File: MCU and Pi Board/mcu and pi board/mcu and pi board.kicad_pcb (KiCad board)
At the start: 4 copper layers, 141.1 x 213.2 mm, 100 parts, among them IC3 CSD17578Q3A, IC4 CSD17578Q3A, J1 PJ-002A, J10 ET60T-D04-0-00-D04-X-R1-S, J11 Conn_02x13_Odd_Even, J12 430450428, J13 IPBT-105-H1-T-D-GP, J14 IPBT-105-H1-T-D-GP, J15 Conn_01x28_Socket, J16 Conn_01x28_Socket, J17 DebugnBoot, J18 UART-PINS, J2 ET60S-D04-3-08-D04-X-R1-S, J22 Conn_01x03_Pin, J23 TB006-508-03BE, J24 TB006-508-03BE, J25 TB006-508-03BE, J3 BM04B-GHS-TBT, J4 PJ-002A, J5 Conn_02x20_Odd_Even, J6 Conn_01x04_Socket, J7 Conn_01x04_Pin, J8 PWM Connector, J9 ESC ADAPTER - BACKPLANE, Q1 BSC010N04LS6ATMA1, Q2 BSC010N04LS6ATMA1, U1 STM32F091CCT6, U2 LM3940IMPX-3.3/NOPB, U3 LTC4370CMS_PBF, U4 TPS40305DRCR, U5 RASPBERRY_PI_4B_4GB, U6 MC74HC157ADR2G, U7 MC74HC157ADR2G

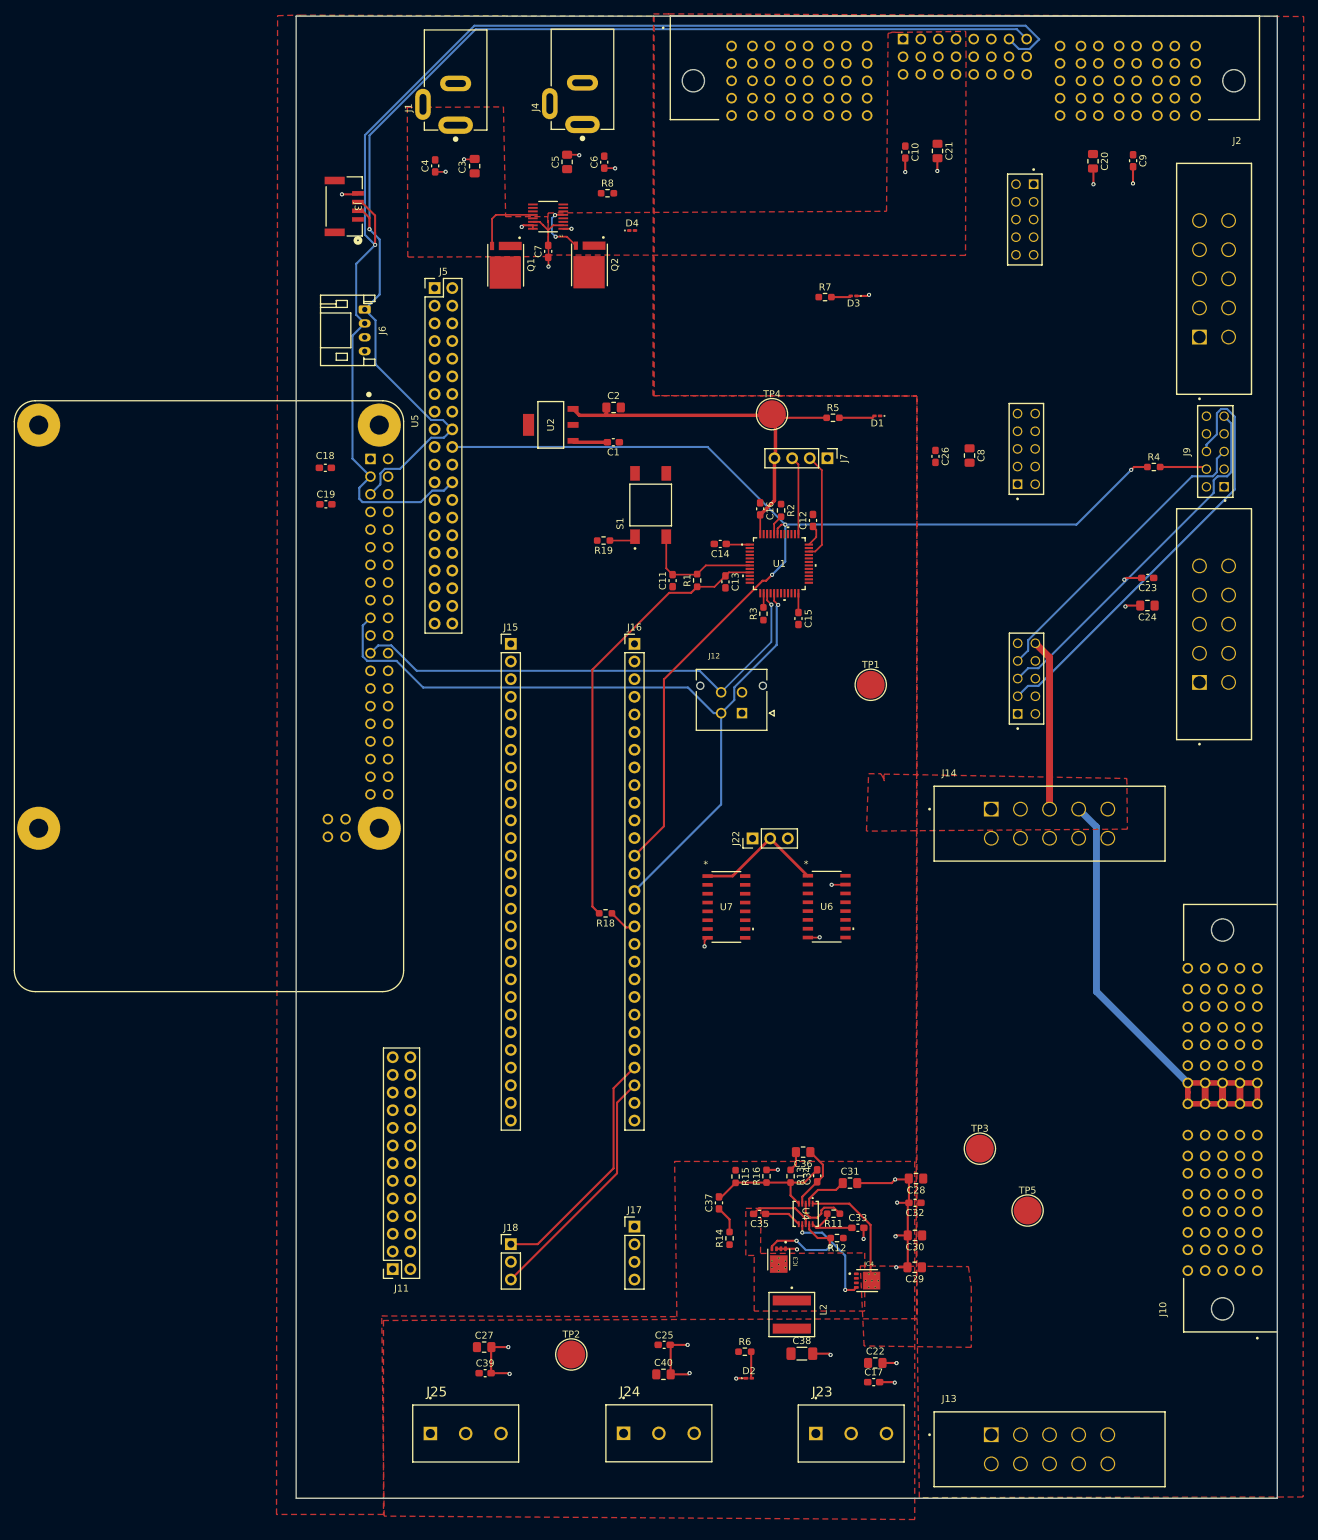
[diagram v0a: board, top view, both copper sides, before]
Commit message: yeet
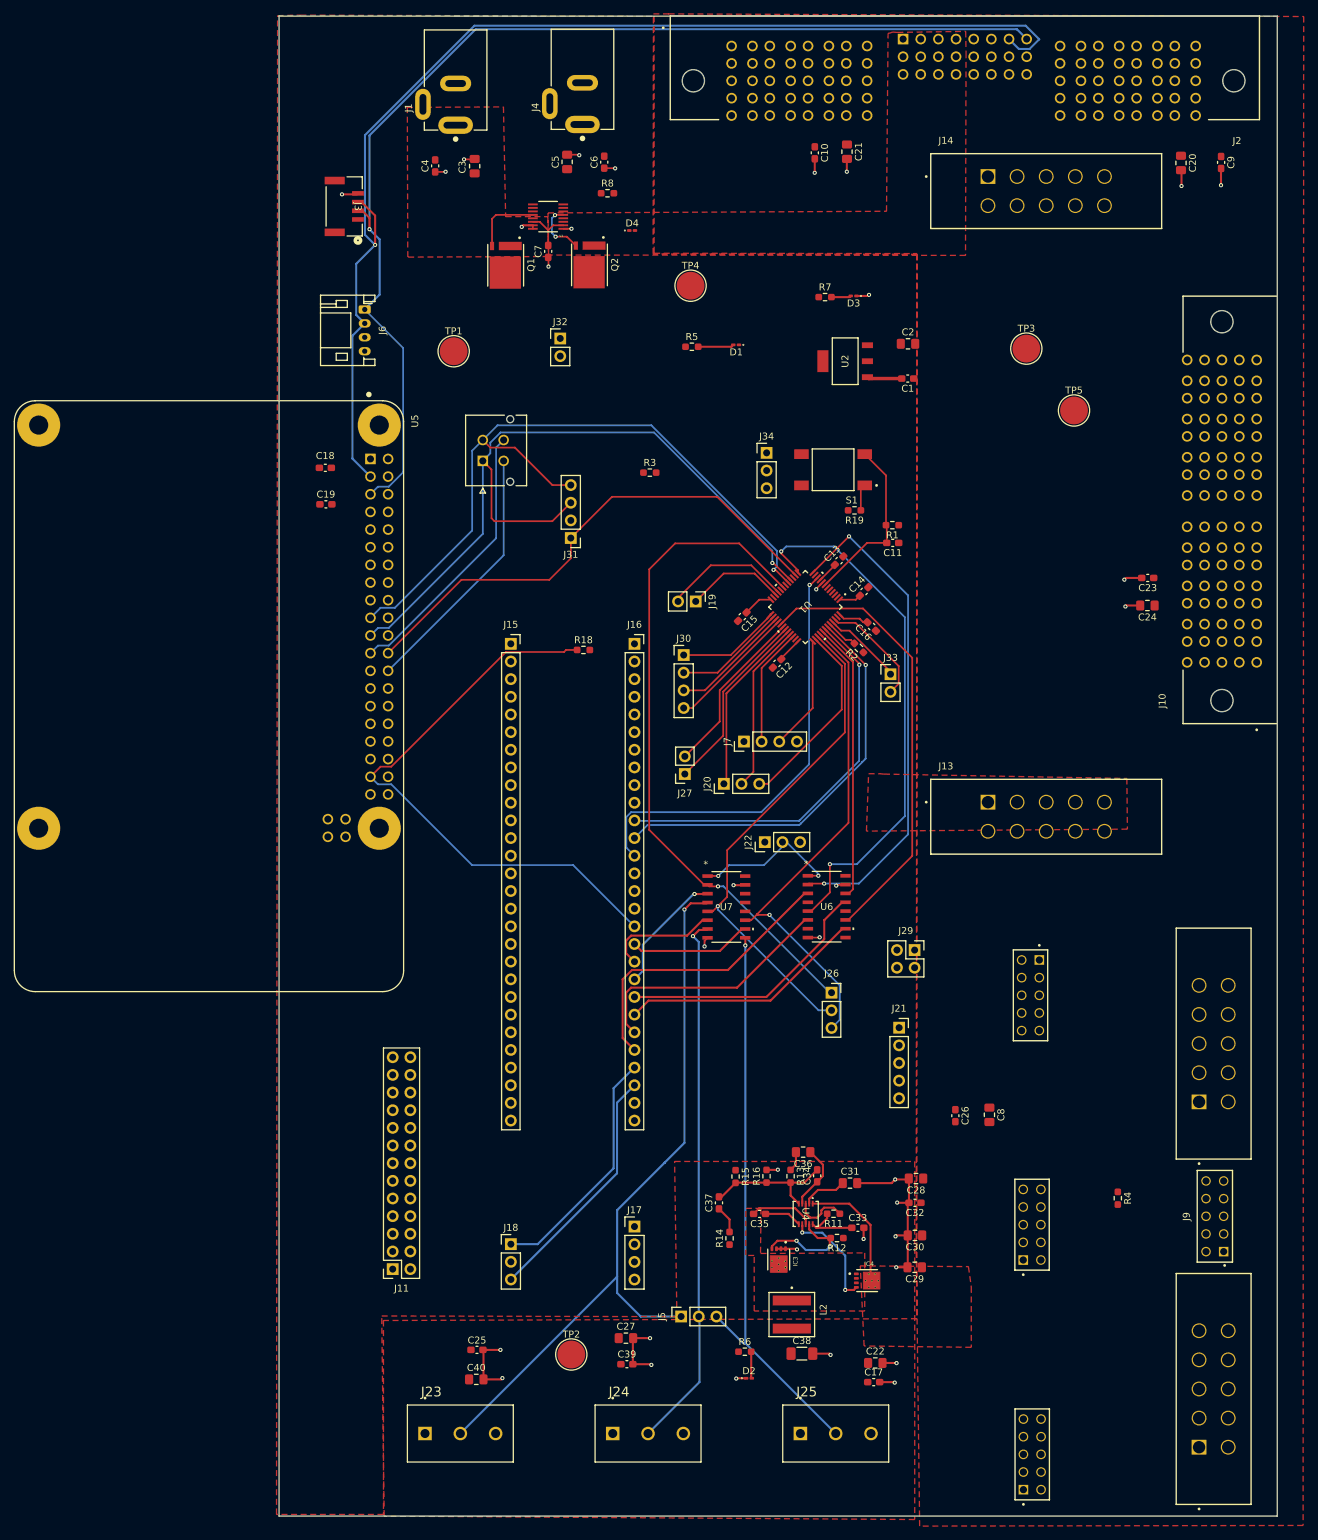
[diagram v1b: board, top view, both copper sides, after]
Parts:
- added J19: Conn_01x02_Pin, Connector_PinHeader_2.54mm:PinHeader_1x02_P2.54mm_Vertical, F.Cu at (218.9, 112.3)
- added J20: Conn_01x03_Pin, Connector_PinHeader_2.54mm:PinHeader_1x03_P2.54mm_Vertical, F.Cu at (223.0, 138.5)
- added J21: Conn_01x05, Connector_PinSocket_2.54mm:PinSocket_1x05_P2.54mm_Vertical, F.Cu at (248.2, 173.6)
- added J26: Conn_01x03_Pin, Connector_PinSocket_2.54mm:PinSocket_1x03_P2.54mm_Vertical, F.Cu at (238.5, 168.6)
- added J27: Conn_01x02_Pin, Connector_PinSocket_2.54mm:PinSocket_1x02_P2.54mm_Vertical, F.Cu at (217.4, 137.1)
- added J29: Conn_02x02_Pin, Connector_PinSocket_2.54mm:PinSocket_2x02_P2.54mm_Vertical, F.Cu at (250.4, 162.4)
- added J30: Conn_01x04_Pin, Connector_PinHeader_2.54mm:PinHeader_1x04_P2.54mm_Vertical, F.Cu at (217.2, 120.0)
- added J31: Conn_01x04_Pin, Connector_PinHeader_2.54mm:PinHeader_1x04_P2.54mm_Vertical, F.Cu at (201.0, 103.2)
- added J32: Conn_01x02_Pin, Connector_PinHeader_2.54mm:PinHeader_1x02_P2.54mm_Vertical, F.Cu at (199.4, 74.5)
- added J33: Conn_01x02_Pin, Connector_PinHeader_2.54mm:PinHeader_1x02_P2.54mm_Vertical, F.Cu at (247.0, 122.8)
- added J34: Conn_01x03_Pin, Connector_PinHeader_2.54mm:PinHeader_1x03_P2.54mm_Vertical, F.Cu at (229.1, 90.9)
- J15, J16: footprint Connector_PinHeader_2.54mm:PinHeader_1x28_P2.54mm_Vertical -> Connector_PinSocket_2.54mm:PinSocket_1x28_P2.54mm_Vertical
- J5: value Conn_02x20_Odd_Even -> Conn_01x03_Pin; footprint Connector_PinHeader_2.54mm:PinHeader_2x20_P2.54mm_Vertical -> Connector_PinSocket_2.54mm:PinSocket_1x03_P2.54mm_Vertical
- TP1, TP2: value 6V -> TestPoint
- TP4: value 3.3V -> TestPoint
- moved J5 152.1 mm to (216.8, 215.2), turned to 90 degrees
- moved TP3 115.3 mm to (266.5, 75.9)
- moved TP5 115.3 mm to (273.4, 84.8)
- moved J8 111.6 mm to (267.3, 202.0)
- moved J9 110.0 mm to (293.5, 200.8)
- moved R4 105.3 mm to (279.7, 198.2), turned to -90 degrees
- moved C26 94.9 mm to (256.3, 186.3)
- moved C8 94.9 mm to (261.2, 186.2)
- moved J13 91.0 mm to (269.4, 143.3)
- moved J14 91.0 mm to (269.4, 53.3)
- moved J10 87.5 mm to (294.6, 99.3)
- moved TP1 76.8 mm to (184.1, 76.3)
- moved J23 56.2 mm to (180.0, 232.0)
- moved J25 53.2 mm to (234.0, 232.0)
- moved J12 52.0 mm to (188.3, 92.1), turned to -90 degrees
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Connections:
- J10 pad P03_1: +12V -> GND
- J10 pad P03_10: +12V -> GND
- J10 pad P03_2: +12V -> GND
- J10 pad P03_3: +12V -> GND
- J10 pad P03_4: +12V -> GND
- J10 pad P03_5: +12V -> GND
- J10 pad P03_6: +12V -> GND
- J10 pad P03_7: +12V -> GND
- J10 pad P03_8: +12V -> GND
- J10 pad P03_9: +12V -> GND
- J10 pad P04_1: +12V -> GND
- J10 pad P04_10: +12V -> GND
- J10 pad P04_2: +12V -> GND
- J10 pad P04_3: +12V -> GND
- J10 pad P04_4: +12V -> GND
- J10 pad P04_5: +12V -> GND
- J10 pad P04_6: +12V -> GND
- J10 pad P04_7: +12V -> GND
- J10 pad P04_8: +12V -> GND
- J10 pad P04_9: +12V -> GND
- J10 pad P07_1: GND -> +12V
- J10 pad P07_10: GND -> +12V
- J10 pad P07_2: GND -> +12V
- J10 pad P07_3: GND -> +12V
- J10 pad P07_4: GND -> +12V
- J10 pad P07_5: GND -> +12V
- J10 pad P07_6: GND -> +12V
- J10 pad P07_7: GND -> +12V
- J10 pad P07_8: GND -> +12V
- J10 pad P07_9: GND -> +12V
- J10 pad P08_1: GND -> +12V
- J10 pad P08_10: GND -> +12V
- J10 pad P08_2: GND -> +12V
- J10 pad P08_3: GND -> +12V
- J10 pad P08_4: GND -> +12V
- J10 pad P08_5: GND -> +12V
- J10 pad P08_6: GND -> +12V
- J10 pad P08_7: GND -> +12V
- J10 pad P08_8: GND -> +12V
- J10 pad P08_9: GND -> +12V
- J5 pad 1: /MCU/NRST -> /servo and esc/SERVO_PWM_0
- J5 pad 2: /MCU/BOOT0 -> /servo and esc/SERVO_PWM_1
- J5 pad 3: /MCU/SWDIO  -> /servo and esc/SERVO_PWM_2
- U1 pad 10: /MCU/PA0 -> /MCU/GPIO13
- U1 pad 19: /MCU/PB1 -> /MCU/STM_SERVO_PWM_0
- U1 pad 2: /MCU/PC13 -> unconnected-(U1A-PC13-Pad2)
- U1 pad 21: /MCU/PB10 -> /MCU/SCL_BREAKOUT
- U1 pad 22: /MCU/PB11 -> /MCU/SDA_BREAKOUT
- U1 pad 25: /MCU/PB12 -> /MCU/CS_BREAKOUT
- U1 pad 26: /MCU/PB13 -> /MCU/SCK_BREAKOUT
- U1 pad 27: /MCU/PB14 -> /MCU/MISO_BREAKOUT
- U1 pad 28: /MCU/PB15 -> /MCU/MOSI_BREAKOUT
- U1 pad 29: /MCU/PA8 -> /MCU/STM_ESC_PWM_2
- U1 pad 3: /MCU/PC14 -> unconnected-(U1A-PC14-OSC32_IN-Pad3)
- U1 pad 39: /MCU/PB3 -> /MCU/STM_SERVO_PWM_1
- U1 pad 4: /MCU/PC15 -> unconnected-(U1A-PC15-OSC32_OUT-Pad4)
- U1 pad 40: /MCU/PB4 -> /MCU/STM_SERVO_PWM_2
- U1 pad 41: /MCU/PB5 -> /MCU/STM_ESC_PWM_3
- U1 pad 43: /MCU/GPIO13 -> /MCU/GPIO14
- U1 pad 46: /MCU/GPIO14 -> /MCU/PB9
- U1 pad 5: /MCU/OSC_IN -> unconnected-(U1A-PF0-OSC_IN-Pad5)
- U1 pad 6: /MCU/PF1 -> unconnected-(U1A-PF1-OSC_OUT-Pad6)
- U5 pad S1: Net-(U5-SHIELD-PadS1) -> unconnected-(U5-SHIELD-PadS1)_2
- U5 pad S2: Net-(U5-SHIELD-PadS1) -> unconnected-(U5-SHIELD-PadS1)_3
- U5 pad S3: Net-(U5-SHIELD-PadS1) -> unconnected-(U5-SHIELD-PadS1)_1
- U5 pad S4: Net-(U5-SHIELD-PadS1) -> unconnected-(U5-SHIELD-PadS1)
- U6 pad 11: /MCU/PA2 -> /MCU/STM_ESC_PWM_2
- U6 pad 14: /MCU/PA3 -> /MCU/STM_ESC_PWM_3
- U6 pad 2: /MCU/PA0 -> /MCU/PA2
- U6 pad 5: /MCU/PA1 -> /MCU/PA3
- U7 pad 11: /MCU/PA10 -> /MCU/STM_SERVO_PWM_2
- U7 pad 2: /MCU/PA8 -> /MCU/STM_SERVO_PWM_0
- U7 pad 5: /MCU/PA9 -> /MCU/STM_SERVO_PWM_1
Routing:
- net +3.3V: track 130.1 -> 18.4 mm
- net /MCU/GPIO12: track 0.00 -> 110.9 mm, vias 0 -> 1
- net +5V: track 110.6 -> 5.02 mm
- net /servo and esc/SERVO_PWM_0: track 0.00 -> 105.2 mm, vias 0 -> 1
- net /MCU/GPIO13: track 167.1 -> 63.0 mm, vias 3 -> 1
- net /MCU/STM_SERVO_PWM_0: track 0.00 -> 96.9 mm, vias 0 -> 1
- net /servo and esc/SERVO_PWM_2: track 0.00 -> 82.4 mm, vias 0 -> 1
- net /MCU/GPIO9: track 4.15 -> 84.2 mm
- net /servo and esc/SERVO_PWM_1: track 0.00 -> 77.4 mm, vias 0 -> 1
- net /MCU/PA3: track 0.00 -> 77.0 mm, vias 0 -> 2
- net /MCU/STM_SERVO_PWM_1: track 0.00 -> 72.6 mm, vias 0 -> 1
- net /MCU/STM_SERVO_PWM_2: track 0.00 -> 72.3 mm, vias 0 -> 1
- net /MCU/PA4: track 2.05 -> 74.3 mm
- net /MCU/PA2: track 0.00 -> 71.2 mm, vias 0 -> 2
- net /MCU/STM_ESC_PWM_2: track 0.00 -> 64.7 mm
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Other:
- board size 141.1 x 213.2 mm -> 143.6 x 215.8 mm
